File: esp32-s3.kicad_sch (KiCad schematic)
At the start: 9 parts, among them SW1 RESET, SW2 BOOT, U3 ESP32-S3-WROOM-1

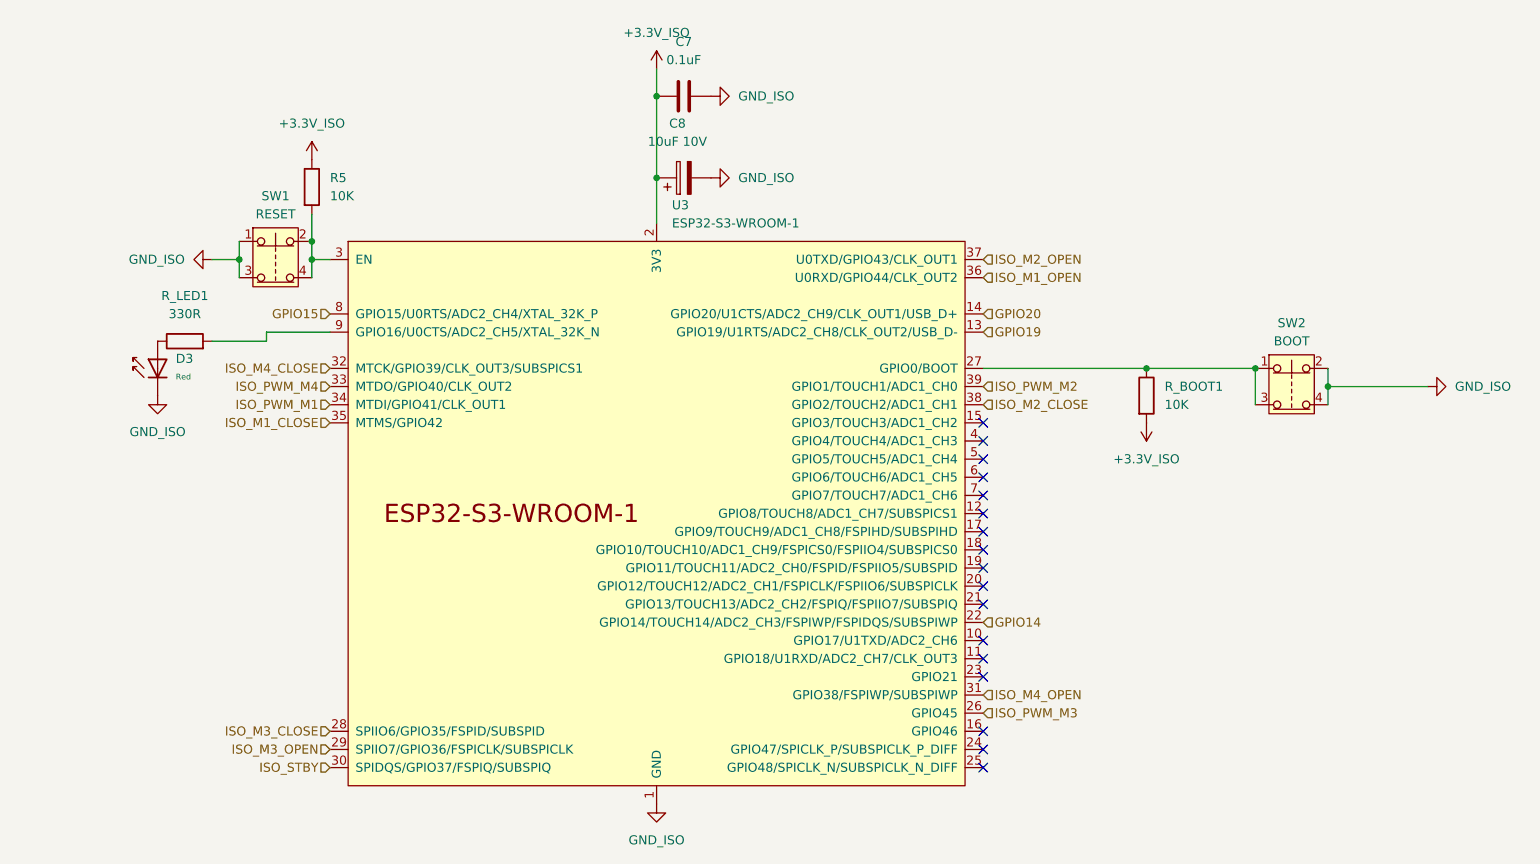
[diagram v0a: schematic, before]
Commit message: V 1.2
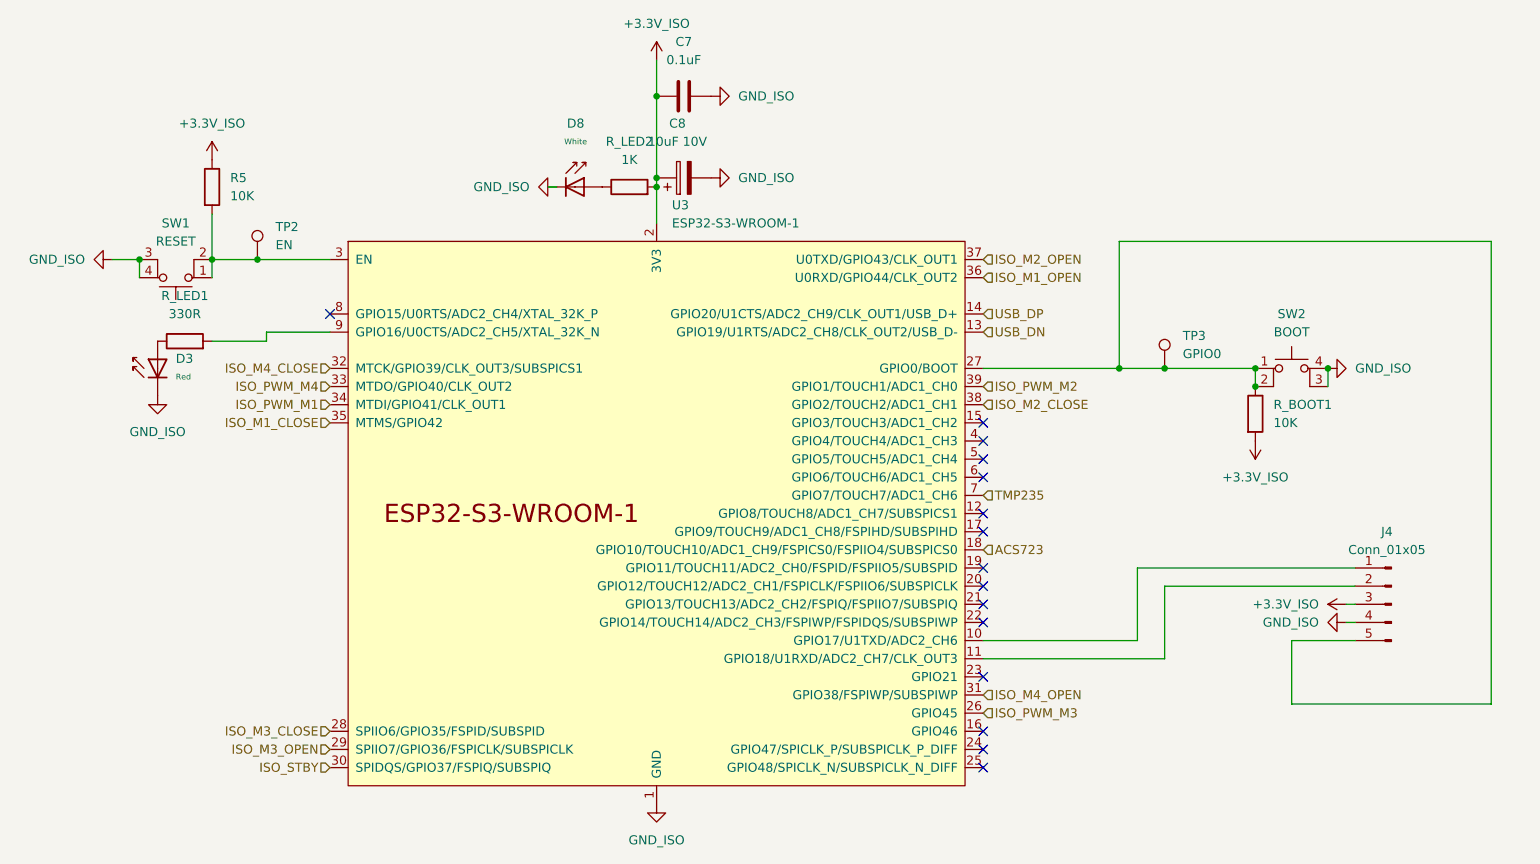
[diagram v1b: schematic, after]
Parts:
- added D8: White, PCM_JLCPCB:D_0805, symbol PCM_JLCPCB-Diodes:LED,0805,Red
- added J4: Conn_01x05, Connector_PinHeader_2.54mm:PinHeader_1x05_P2.54mm_Vertical, symbol Connector:Conn_01x05_Pin
- added R_LED2: 1K, Resistor_SMD:R_0603_1608Metric, symbol Device:R
- added TP2: EN, barn_shade_controller:TestPoint_Pad_D1.0mm_No_SolderMask, symbol Connector:TestPoint
- added TP3: GPIO0, barn_shade_controller:TestPoint_Pad_D1.0mm_No_SolderMask, symbol Connector:TestPoint
- SW1, SW2: symbol Switch:SW_Push_Open_Dual -> Switch:SW_MEC_5E
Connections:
- net +3.3V_ISO: now also J4.3 (Pin_3), R_LED2.2
- net GND_ISO: now also SW1.4 (A), SW2.3 (K), D8.1, J4.4 (Pin_4); no longer SW1.1, SW2.2
- net at R5.2, SW1.2, U3.3 (EN): now also SW1.1, TP2.1; no longer SW1.4
- net at U3.10 (GPIO17/U1TXD/ADC2_CH6): now also J4.1 (Pin_1)
- net at U3.11 (GPIO18/U1RXD/ADC2_CH7/CLK_OUT3): now also J4.2 (Pin_2)
- net ACS723: now reaches U3.18 (GPIO10/TOUCH10/ADC1_CH9/FSPICS0/FSPIIO4/SUBSPICS0)
- net at R_BOOT1.1, SW2.1, U3.27 (GPIO0/BOOT): now also SW2.2, J4.5 (Pin_5), TP3.1; no longer SW2.3
- net TMP235: now reaches U3.7 (GPIO7/TOUCH7/ADC1_CH6)
- net GPIO14: no longer names the net of U3.22 (GPIO14/TOUCH14/ADC2_CH3/FSPIWP/FSPIDQS/SUBSPIWP)
- net GPIO15: no longer names the net of U3.8 (GPIO15/U0RTS/ADC2_CH4/XTAL_32K_P)
- net GPIO19 renamed USB_DN
- net GPIO20 renamed USB_DP
- new net: D8.2, R_LED2.1
- no-connect marks 17 -> 15
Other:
- moved on the sheet: R5, R_BOOT1
